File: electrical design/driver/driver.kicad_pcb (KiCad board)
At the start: 2 copper layers, 38 x 45 mm, 18 parts, among them J1 XT30PW-F, J2 PH2.0 6P, J3 SH1.0 8P, Q1 IRFR5410PbF, U1 VNH5050A-E

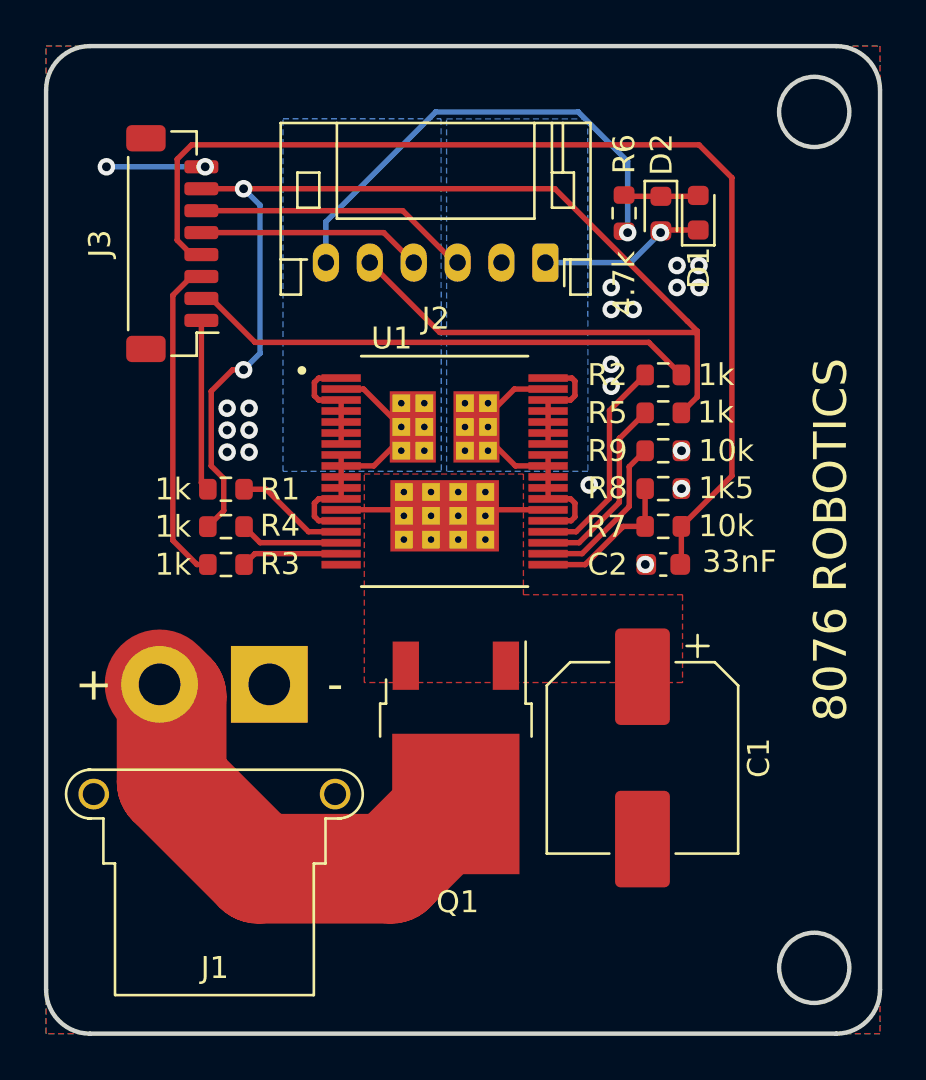
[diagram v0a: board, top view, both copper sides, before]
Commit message: submit all pcbs for production
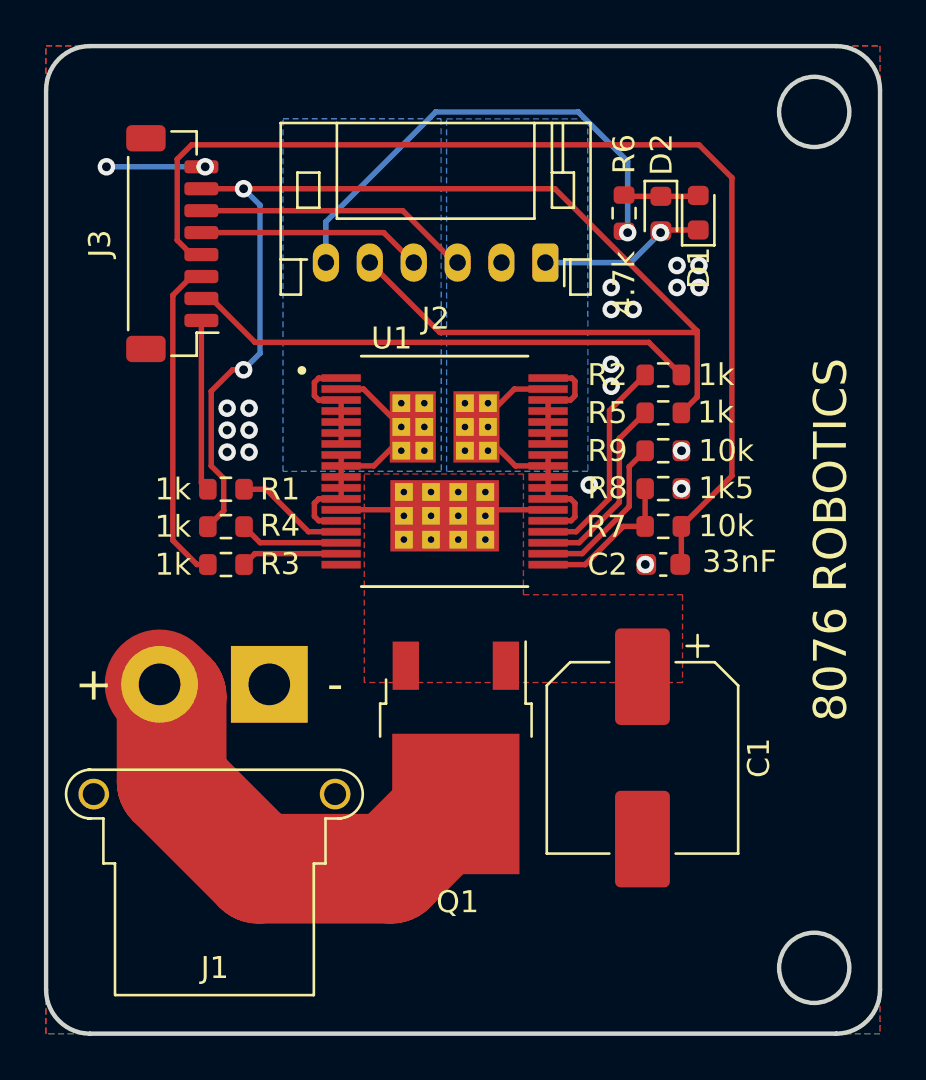
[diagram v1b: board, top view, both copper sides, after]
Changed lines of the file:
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@@
       (layerselection 0x00010fc_ffffffff)
       (disableapertmacros false)
-      (usegerberextensions false)
+      (usegerberextensions true)
       (usegerberattributes true)
-      (usegerberadvancedattributes true)
-      (creategerberjobfile true)
+      (usegerberadvancedattributes false)
+      (creategerberjobfile false)
       (svguseinch false)
       (svgprecision 6)
@@
       (plotinvisibletext false)
       (sketchpadsonfab false)
-      (subtractmaskfromsilk false)
+      (subtractmaskfromsilk true)
       (outputformat 1)
       (mirror false)
-      (drillshape 1)
+      (drillshape 0)
       (scaleselection 1)
-      (outputdirectory "")
+      (outputdirectory "fab/")
     )
   )
@@
     (pad "8" smd roundrect (at 3.5 1.325 90) (size 0.6 1.55) (layers "F.Cu" "F.Paste" "F.Mask") (roundrect_rratio 0.25)
       (net 2 "GND") (pinfunction "Pin_8") (pintype "passive"))
-    (pad "MP" smd roundrect (at 4.8 -1.2 90) (size 1.2 1.8) (layers "F.Cu" "F.Paste" "F.Mask") (roundrect_rratio 0.208333))
-    (pad "MP" smd roundrect (at -4.8 -1.2 90) (size 1.2 1.8) (layers "F.Cu" "F.Paste" "F.Mask") (roundrect_rratio 0.208333))
+    (pad "MP" smd roundrect (at 4.8 -1.2 90) (size 1.2 1.8) (layers "F.Cu" "F.Paste" "F.Mask") (roundrect_rratio 0.2083333333))
+    (pad "MP" smd roundrect (at -4.8 -1.2 90) (size 1.2 1.8) (layers "F.Cu" "F.Paste" "F.Mask") (roundrect_rratio 0.2083333333))
     (model "${KICAD6_3DMODEL_DIR}/Connector_JST.3dshapes/JST_SH_BM08B-SRSS-TB_1x08-1MP_P1.00mm_Vertical.wrl"
       (offset (xyz 0 0 0))
@@
   (segment (start 121.9207 98.988212) (end 121.9207 99.0793) (width 0.25) (layer "F.Cu") (net 9))
   (segment (start 101.25 92.5) (end 115.432488 92.5) (width 0.25) (layer "F.Cu") (net 9))
-  (segment (start 121.466244 98.533756) (end 121.9207 98.988212) (width 0.25) (layer "F.Cu") (net 9))
+  (segment (start 115.432488 92.5) (end 121.9207 98.988212) (width 0.25) (layer "F.Cu") (net 9))
   (segment (start 99.775 101.725) (end 100.75 100.75) (width 0.25) (layer "F.Cu") (net 9))
   (segment (start 121.9207 101.98735) (end 121.1957 102.71235) (width 0.25) (layer "F.Cu") (net 9))
@@
   (segment (start 99.325 92.5) (end 101.25 92.5) (width 0.25) (layer "F.Cu") (net 9))
   (segment (start 100.75 100.75) (end 101.25 100.75) (width 0.25) (layer "F.Cu") (net 9))
-  (segment (start 115.432488 92.5) (end 121.466244 98.533756) (width 0.25) (layer "F.Cu") (net 9))
   (segment (start 99.775 105.130988) (end 99.775 101.725) (width 0.25) (layer "F.Cu") (net 9))
   (segment (start 99.6207 107.89595) (end 100.3457 107.17095) (width 0.25) (layer "F.Cu") (net 9))
   (segment (start 107 95.86375) (end 110.18625 99.05) (width 0.25) (layer "F.Cu") (net 9))
   (segment (start 100.3457 105.701688) (end 99.775 105.130988) (width 0.25) (layer "F.Cu") (net 9))
-  (segment (start 99.6207 107.89595) (end 99.60405 107.89595) (width 0.25) (layer "F.Cu") (net 9))
-  (segment (start 99.60405 107.89595) (end 99.5 108) (width 0.25) (layer "F.Cu") (net 9))
   (segment (start 100.3457 107.17095) (end 100.3457 105.701688) (width 0.25) (layer "F.Cu") (net 9))
   (via (at 101.25 100.75) (size 0.8) (drill 0.4) (layers "F.Cu" "B.Cu") (net 9))
